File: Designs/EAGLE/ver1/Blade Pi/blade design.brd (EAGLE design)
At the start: 114.3 x 91.1 mm, 35 parts

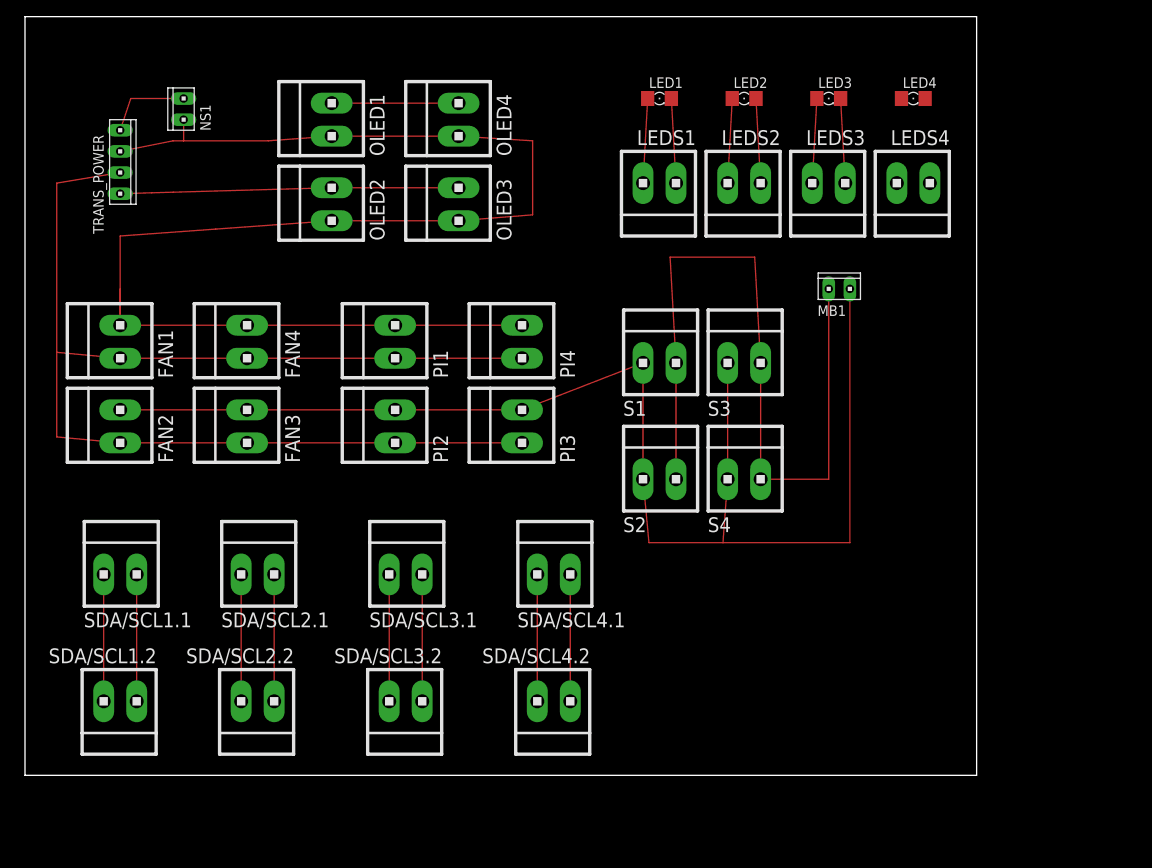
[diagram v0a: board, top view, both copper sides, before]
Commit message: First design complete
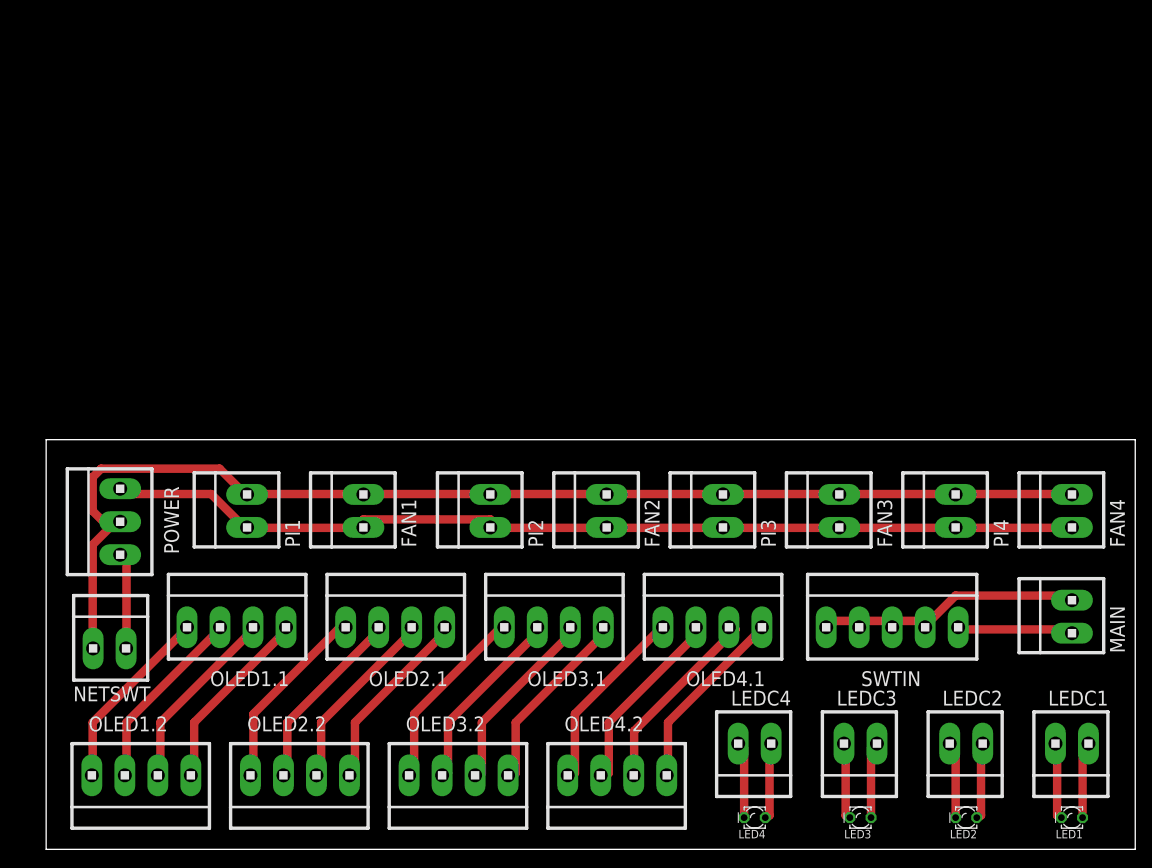
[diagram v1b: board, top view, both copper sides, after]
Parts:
- removed LEDS1, LEDS2, LEDS3, LEDS4, OLED1, OLED2, OLED3, OLED4, S1, S2, S3, S4, SDA/SCL1.1, SDA/SCL1.2, SDA/SCL2.1, SDA/SCL2.2, SDA/SCL3.1, SDA/SCL3.2, SDA/SCL4.1, SDA/SCL4.2: (no value), con-amp:1X2MTA
- removed MB1, NS1: (no value), con-amp:10X02MTA
- removed TRANS_POWER: (no value), con-amp:10X04MTA
- added LEDC1, LEDC2, LEDC3, LEDC4, MAIN, NETSWT: (no value), con-amp:1X2MTA
- added OLED1.1, OLED1.2, OLED2.1, OLED2.2, OLED3.1, OLED3.2, OLED4.1, OLED4.2: (no value), con-amp:1X4MTA
- added POWER: (no value), con-amp:1X3MTA
- added SWTIN: (no value), con-amp:1X5MTA
- LED1, LED2, LED3, LED4: device eagle-ltspice:LED_1206 -> eagle-ltspice:LED_LD260
- moved FAN4 101.1 mm to (125.7, 40.6)
- moved LED1 99.6 mm to (125.7, 3.81), turned to 180 degrees
- moved LED2 90.4 mm to (113.0, 3.81), turned to 180 degrees
- moved LED4 88.4 mm to (87.6, 3.81), turned to 180 degrees
- moved LED3 86.4 mm to (100.3, 3.81), turned to 180 degrees
- moved FAN3 71.8 mm to (97.8, 40.6)
- moved FAN2 59.3 mm to (69.8, 40.6)
- moved PI4 55.9 mm to (111.8, 40.6)
- moved FAN1 35.6 mm to (40.6, 40.6)
- moved PI1 27.0 mm to (26.7, 40.6)
- moved PI3 26.2 mm to (83.8, 40.6)
- moved PI2 15.3 mm to (55.9, 40.6)
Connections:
- removed net N$10: SDA/SCL3.1.2, SDA/SCL3.2.1
- removed net N$11: SDA/SCL4.1.1, SDA/SCL4.2.2
- removed net N$12: SDA/SCL4.1.2, SDA/SCL4.2.1
- removed net N$14: LED1.C, LEDS1.2
- removed net N$15: LED1.A, LEDS1.1
- removed net N$16: LED2.C, LEDS2.2
- removed net N$17: LED2.A, LEDS2.1
- removed net N$18: LED3.C, LEDS3.2
- removed net N$20: LED4.C, LEDS4.2
- removed net N$21: LED4.A, LEDS4.1
- removed net N$22: LED3.A, LEDS3.1
- removed net N$9: SDA/SCL3.1.1, SDA/SCL3.2.2
- removed net PS: MB1.2, S1.1, S2.1, S3.1, S4.1
- new net GND1: OLED1.1.1, OLED1.2.4
- new net GND2: OLED2.1.1, OLED2.2.4
- new net GND3: OLED3.1.1, OLED3.2.4
- new net GND4: OLED4.1.1, OLED4.2.4
- new net N$1: LED1.K, LEDC1.1
- new net N$3: LED2.K, LEDC2.1
- new net N$4: LED2.A, LEDC2.2
- new net N$5: LED3.K, LEDC3.1
- new net SCL1: OLED1.1.3, OLED1.2.2
- new net SCL2: OLED2.1.3, OLED2.2.2
- new net SCL3: OLED3.1.3, OLED3.2.2
- new net SCL4: OLED4.1.3, OLED4.2.2
- new net SDA1: OLED1.1.4, OLED1.2.1
- new net SDA2: OLED2.1.4, OLED2.2.1
- new net SDA3: OLED3.1.4, OLED3.2.1
- new net SDA4: OLED4.1.4, OLED4.2.1
- new net SWTCH: MAIN.1, SWTIN.2, SWTIN.3, SWTIN.4, SWTIN.5
- new net VCC1: OLED1.1.2, OLED1.2.3
- new net VCC2: OLED2.1.2, OLED2.2.3
- new net VCC3: OLED3.1.2, OLED3.2.3
- new net VCC4: OLED4.1.2, OLED4.2.3
- net 12V: now also NETSWT.1, POWER.3; no longer NS1.1, TRANS_POWER.4
- net 3.3V: now also MAIN.2, SWTIN.1; no longer OLED1.1, OLED2.1, OLED3.1, OLED4.1, TRANS_POWER.1
- net 5V: now also POWER.1; no longer TRANS_POWER.2
- net GND: now also NETSWT.2, POWER.2; no longer MB1.1, NS1.2, OLED1.2, OLED2.2, OLED3.2, OLED4.2, S1.2, S2.2, S3.2, S4.2, TRANS_POWER.3
- net N$2: now also LED1.A, LEDC1.2; no longer SDA/SCL1.1.1, SDA/SCL1.2.2
- net N$6: now also LED3.A, LEDC3.2; no longer SDA/SCL1.1.2, SDA/SCL1.2.1
- net N$7: now also LED4.K, LEDC4.1; no longer SDA/SCL2.1.1, SDA/SCL2.2.2
- net N$8: now also LED4.A, LEDC4.2; no longer SDA/SCL2.1.2, SDA/SCL2.2.1
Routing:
- net GND: track 335.8 -> 145.0 mm
- net PS: track 94.6 -> 0.00 mm
- net 3.3V: track 55.9 -> 13.8 mm
- net SWTCH: track 0.00 -> 33.9 mm
- net 5V: track 150.0 -> 118.3 mm
- net SCL4: track 0.00 -> 23.7 mm
- net GND3: track 0.00 -> 23.6 mm
- net VCC4: track 0.00 -> 23.4 mm
- net VCC3: track 0.00 -> 23.4 mm
- net SCL3: track 0.00 -> 23.2 mm
- net GND2: track 0.00 -> 23.1 mm
- net VCC2: track 0.00 -> 22.9 mm
- net SDA2: track 0.00 -> 22.9 mm
- net SDA4: track 0.00 -> 22.9 mm
- net SDA3: track 0.00 -> 22.8 mm
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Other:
- board size 114.3 x 91.1 mm -> 130.8 x 49.2 mm

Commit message: design commit
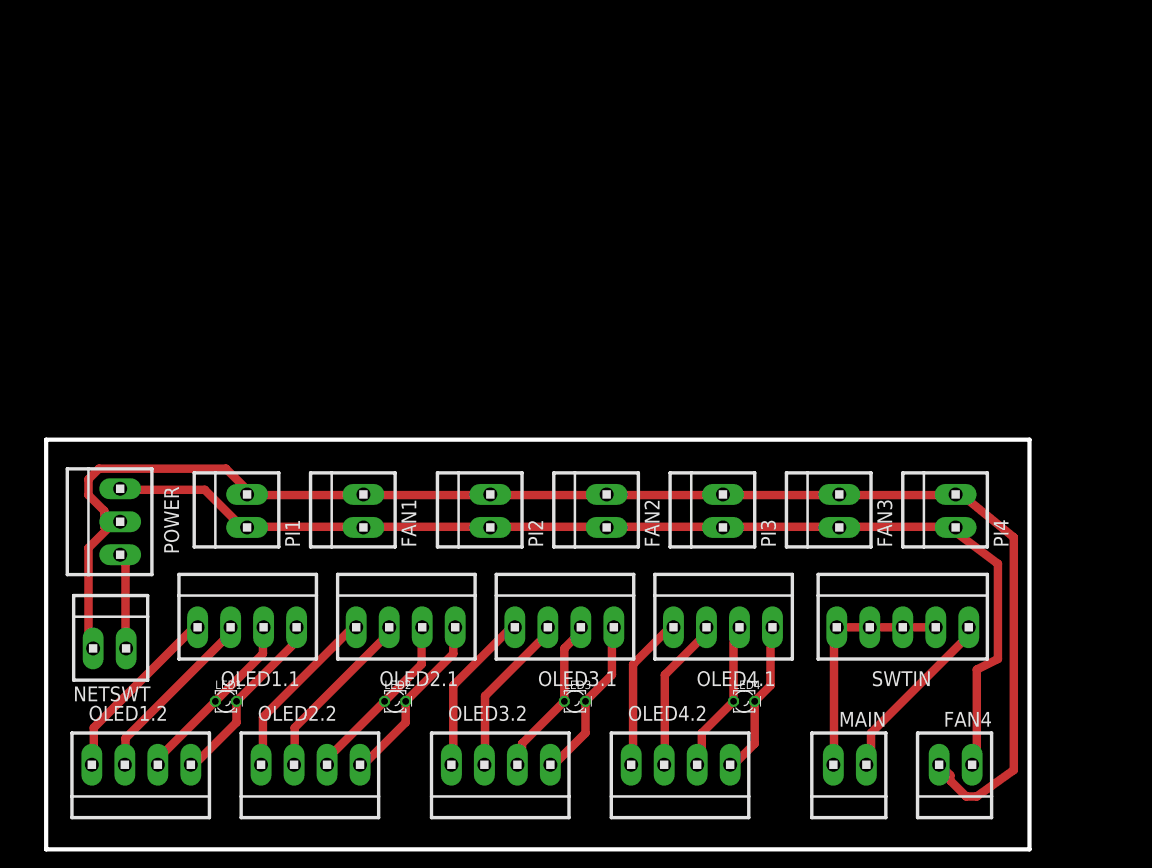
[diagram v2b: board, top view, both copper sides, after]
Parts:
- removed LEDC1, LEDC2, LEDC3, LEDC4: (no value), con-amp:1X2MTA
- moved LED1 102.6 mm to (24.1, 17.8), turned to 0 degrees
- moved LED2 70.0 mm to (44.5, 17.8), turned to 0 degrees
- moved LED3 37.0 mm to (66.0, 17.8), turned to 0 degrees
- moved FAN4 33.5 mm to (111.8, 10.2), turned to 180 degrees
- moved MAIN 32.1 mm to (99.1, 10.2), turned to 180 degrees
- moved LED4 14.0 mm to (86.4, 17.8), turned to 0 degrees
- moved OLED4.2 7.73 mm to (78.7, 10.2)
- moved OLED3.2 5.24 mm to (57.1, 10.2)
- moved OLED2.2 1.80 mm to (34.3, 10.2)
- moved OLED1.1 1.27 mm to (26.7, 26.7)
- moved OLED1.2 1.27 mm to (14.0, 10.2)
- moved OLED2.1 1.27 mm to (45.7, 26.7)
- moved OLED3.1 1.27 mm to (64.8, 26.7)
- moved OLED4.1 1.27 mm to (83.8, 26.7)
- moved SWTIN 1.27 mm to (105.4, 26.7)
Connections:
- removed net N$1: LED1.K, LEDC1.1
- removed net N$2: LED1.A, LEDC1.2
- removed net N$3: LED2.K, LEDC2.1
- removed net N$4: LED2.A, LEDC2.2
- removed net N$5: LED3.K, LEDC3.1
- removed net N$6: LED3.A, LEDC3.2
- removed net N$7: LED4.K, LEDC4.1
- removed net N$8: LED4.A, LEDC4.2
- net GND1: now also LED1.K
- net GND2: now also LED2.K
- net GND3: now also LED3.K
- net GND4: now also LED4.K
- net VCC1: now also LED1.A
- net VCC2: now also LED2.A
- net VCC3: now also LED3.A
- net VCC4: now also LED4.A
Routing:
- net GND: track 145.0 -> 182.9 mm
- net 5V: track 118.3 -> 136.8 mm
- net N$7: track 9.26 -> 0.00 mm
- net N$6: track 9.26 -> 0.00 mm
- net N$3: track 9.26 -> 0.00 mm
- net N$2: track 9.26 -> 0.00 mm
- net N$4: track 9.24 -> 0.00 mm
- net N$5: track 9.24 -> 0.00 mm
- net N$8: track 9.24 -> 0.00 mm
- net N$1: track 9.24 -> 0.00 mm
- net 3.3V: track 13.8 -> 22.1 mm
- net SWTCH: track 33.9 -> 28.8 mm
- net SCL4: track 23.7 -> 19.0 mm
- net VCC4: track 23.4 -> 19.0 mm
- net SDA4: track 22.9 -> 19.0 mm
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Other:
- board size 130.8 x 49.2 mm -> 118.1 x 49.2 mm
